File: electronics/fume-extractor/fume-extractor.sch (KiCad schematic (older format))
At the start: 5 parts

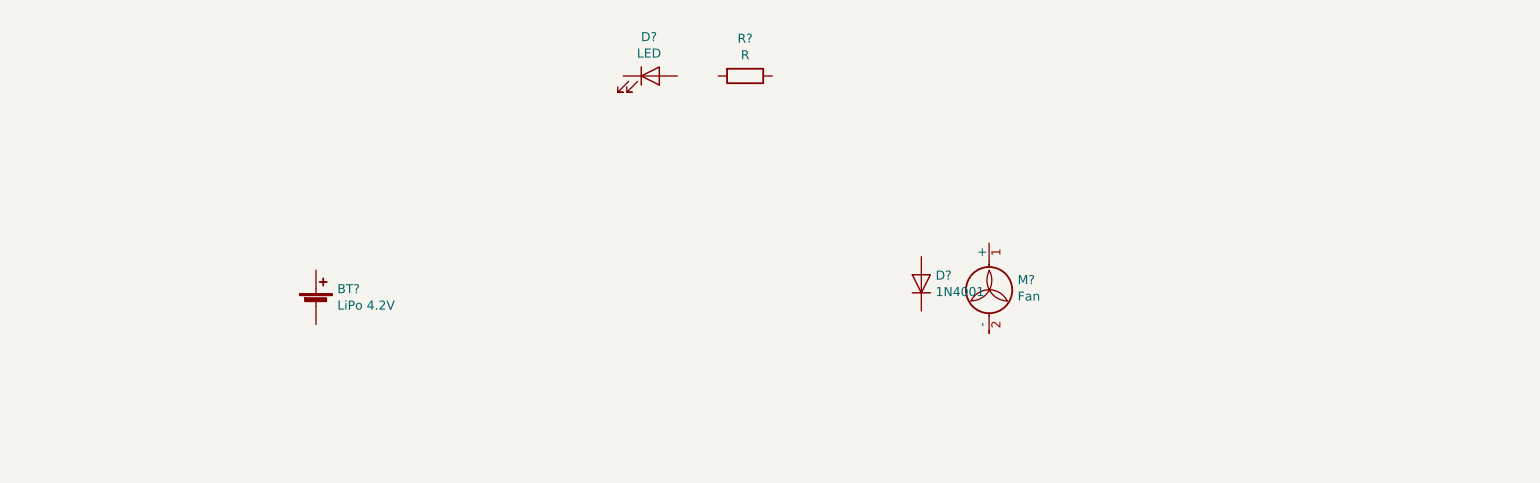
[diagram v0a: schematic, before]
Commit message: schematics finished
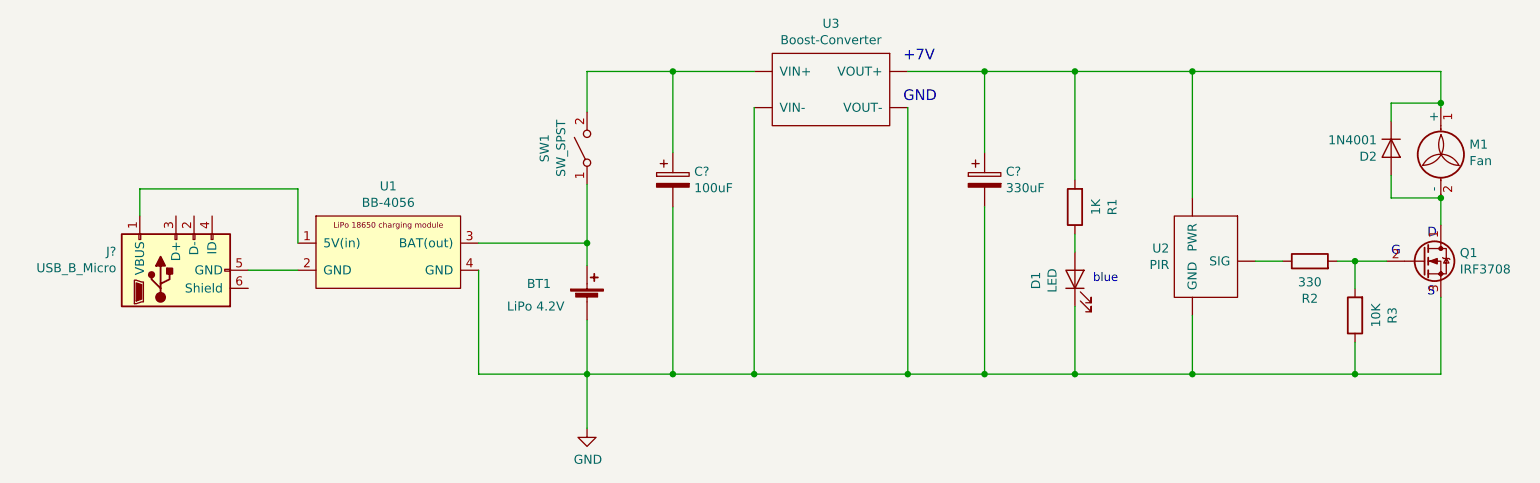
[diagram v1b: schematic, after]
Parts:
- added C?: 330uF, symbol Device:CP
- added C?: 100uF, symbol Device:CP
- added J?: USB_B_Micro, symbol Connector:USB_B_Micro
- added Q1: IRF3708, symbol Device:Q_NMOS_DGS
- added R2: 330, symbol Device:R
- added R3: 10K, symbol Device:R
- added SW1: SW_SPST, symbol Switch:SW_SPST
- added U1: BB-4056, symbol My_Library:BB-4056
- added U2: PIR, symbol My_Library:PIR
- added U3: Boost-Converter, symbol My_Library:Boost-Converter
- R1: renamed from R?; value R -> 1K
- gave numbers to parts that had none: 4
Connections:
- net at BT1.1 (+): now also SW1.1 (A), U1.3 (BAT(out))
- net GND: now reaches BT1.2 (-)
- net GND: now also D1.1 (K), C?.2, C?.2, Q1.3 (S), R3.1, U1.4 (GND), U2.~ (SIG), U3.~ (VOUT-)
- net at M1.1 (+): now also D2.1 (K), R1.2, C?.1, U2.~ (SIG), U3.~ (VOUT-)
- net at M1.2 (-): now also D2.2 (A), Q1.1 (D)
- net at D1.2 (A): now also R1.1
- new net: C?.1, SW1.2 (B), U3.~ (VOUT-)
- new net: Q1.2 (G), R2.2, R3.2
- new net: R2.1, U2.~ (SIG)
- new net: J?.1 (VBUS), U1.1 (5V(in))
- new net: J?.5 (GND), U1.2 (GND)
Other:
- note added: "+7V"
- note added: "D"
- note added: "G"
- note added: "GND"
- note added: "S"
- note added: "blue"
- moved on the sheet: BT1, D1, D2, M1, R1
